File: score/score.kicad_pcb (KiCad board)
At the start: 2 copper layers, 62 x 46 mm, 47 parts, among them J1 Conn_01x02, P8 CONN_01X07, P9 CONN_01X07, U1 74HC595T16-13, U2 HDSP-C8A1, U3 HDSP-C8A1, U4 HDSP-C8A1, U5 74HC595T16-13, U6 74HC595T16-13, U7 TSR1-2433

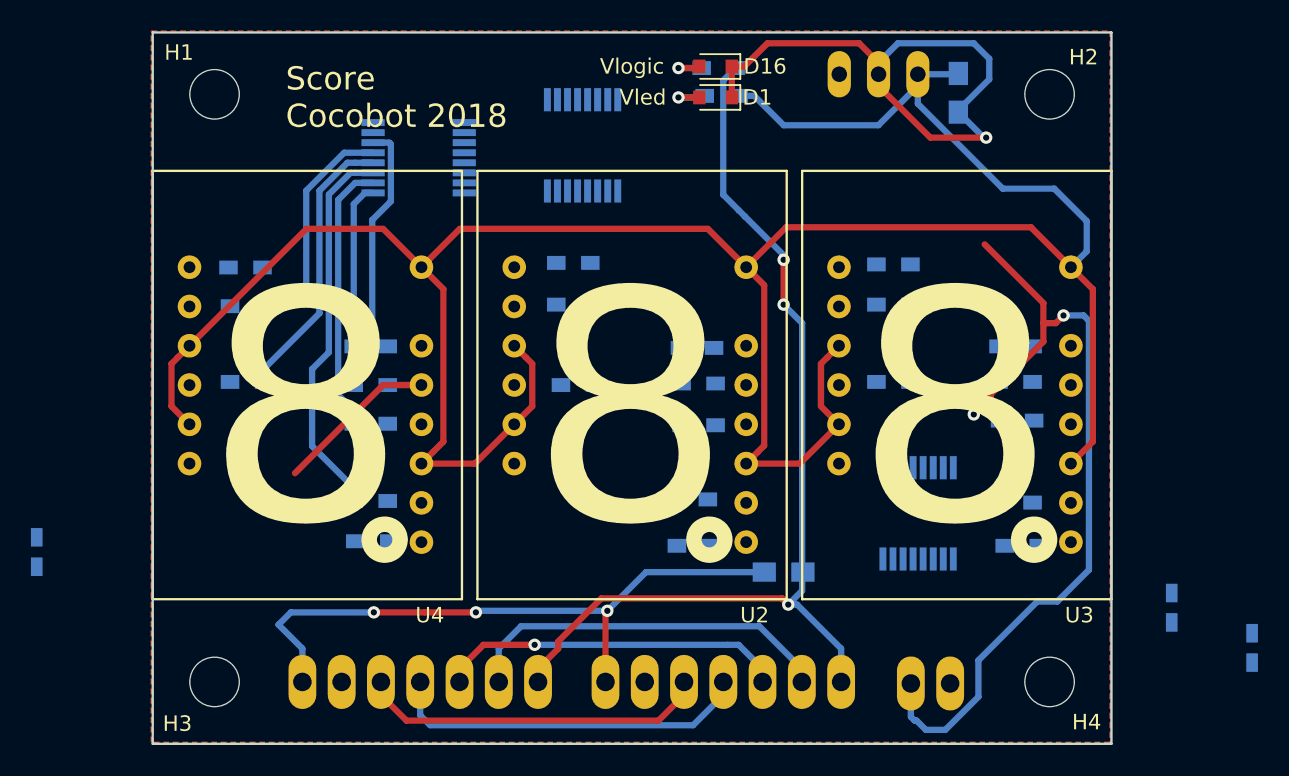
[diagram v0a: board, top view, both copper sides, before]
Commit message: score board routed
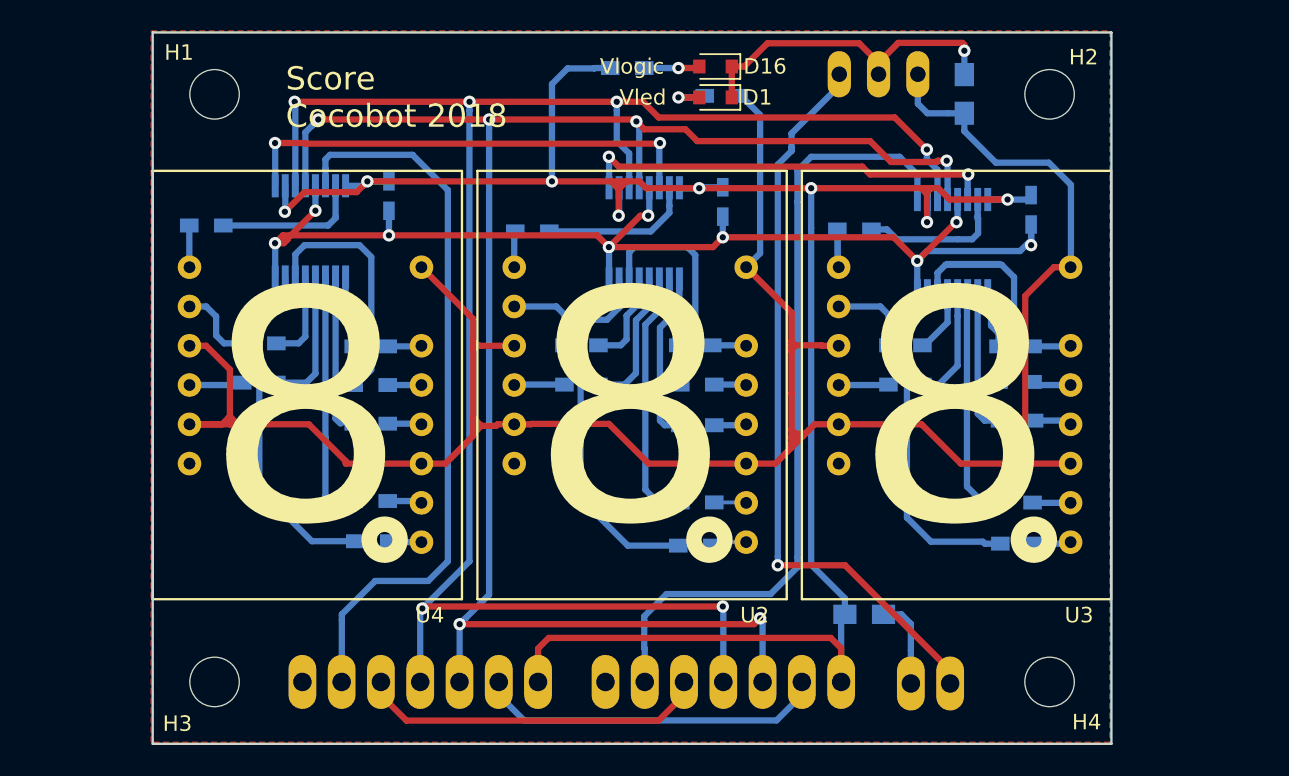
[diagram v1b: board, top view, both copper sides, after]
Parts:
- moved C3 39.1 mm to (86.9, 61.0)
- moved C2 32.4 mm to (65.3, 60.6)
- moved C4 31.7 mm to (106.8, 61.5)
- moved U6 17.5 mm to (101.7, 63.8), turned to 90 degrees
- moved U1 8.47 mm to (60.2, 62.9), turned to 90 degrees
- moved U5 6.95 mm to (81.8, 63.0)
- moved R1 5.91 mm to (80.7, 52.3), turned to 0 degrees
- moved C1 5.88 mm to (96.0, 87.6), turned to 0 degrees
- moved R3 3.71 mm to (53.5, 62.5)
- moved R7 3.39 mm to (95.4, 62.7)
- moved R5 3.34 mm to (74.5, 62.9)
- moved R14 2.74 mm to (98.7, 70.2)
- moved R12 2.68 mm to (77.7, 70.2)
- moved R10 2.53 mm to (56.9, 70.1)
- moved R8 0.80 mm to (98.7, 72.8)
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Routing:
- net /sck_3v3: track 23.7 -> 120.8 mm, vias 0 -> 6
- net /set_output_3v3: track 22.6 -> 114.9 mm, vias 1 -> 7
- net +3V3: track 66.1 -> 136.3 mm, vias 3 -> 8
- net Net-(P9-Pad6): track 0.00 -> 51.3 mm
- net Net-(J1-Pad1): track 0.00 -> 48.5 mm, vias 0 -> 1
- net /mosi_3v3: track 0.00 -> 47.3 mm
- net Net-(U1-Pad9): track 0.00 -> 30.6 mm, vias 0 -> 2
- net GND: track 133.4 -> 105.1 mm, vias 6 -> 10
- net Net-(U5-Pad9): track 0.00 -> 27.4 mm, vias 0 -> 2
- net /ch19_3v3: track 0.00 -> 26.1 mm
- net /ch15_3v3: track 0.00 -> 24.7 mm
- net /ch7_3v3: track 0.00 -> 22.0 mm
- net /ch23_3v3: track 0.00 -> 22.0 mm
- net /ch22_3v3: track 0.00 -> 19.8 mm
- net +3.3VP: track 175.2 -> 157.2 mm
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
